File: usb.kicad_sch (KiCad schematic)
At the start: 17 parts, among them J3 USB_C_Receptacle_USB2.0_14P, J4 USB_C_Receptacle_USB2.0_14P, J5 USB_C_Receptacle_USB2.0_14P, U1 ECP5U_12_CABGA256, U5 TPD2EUSB30, U6 TPD2EUSB30, U7 FT231XQ, U8 TPD2EUSB30

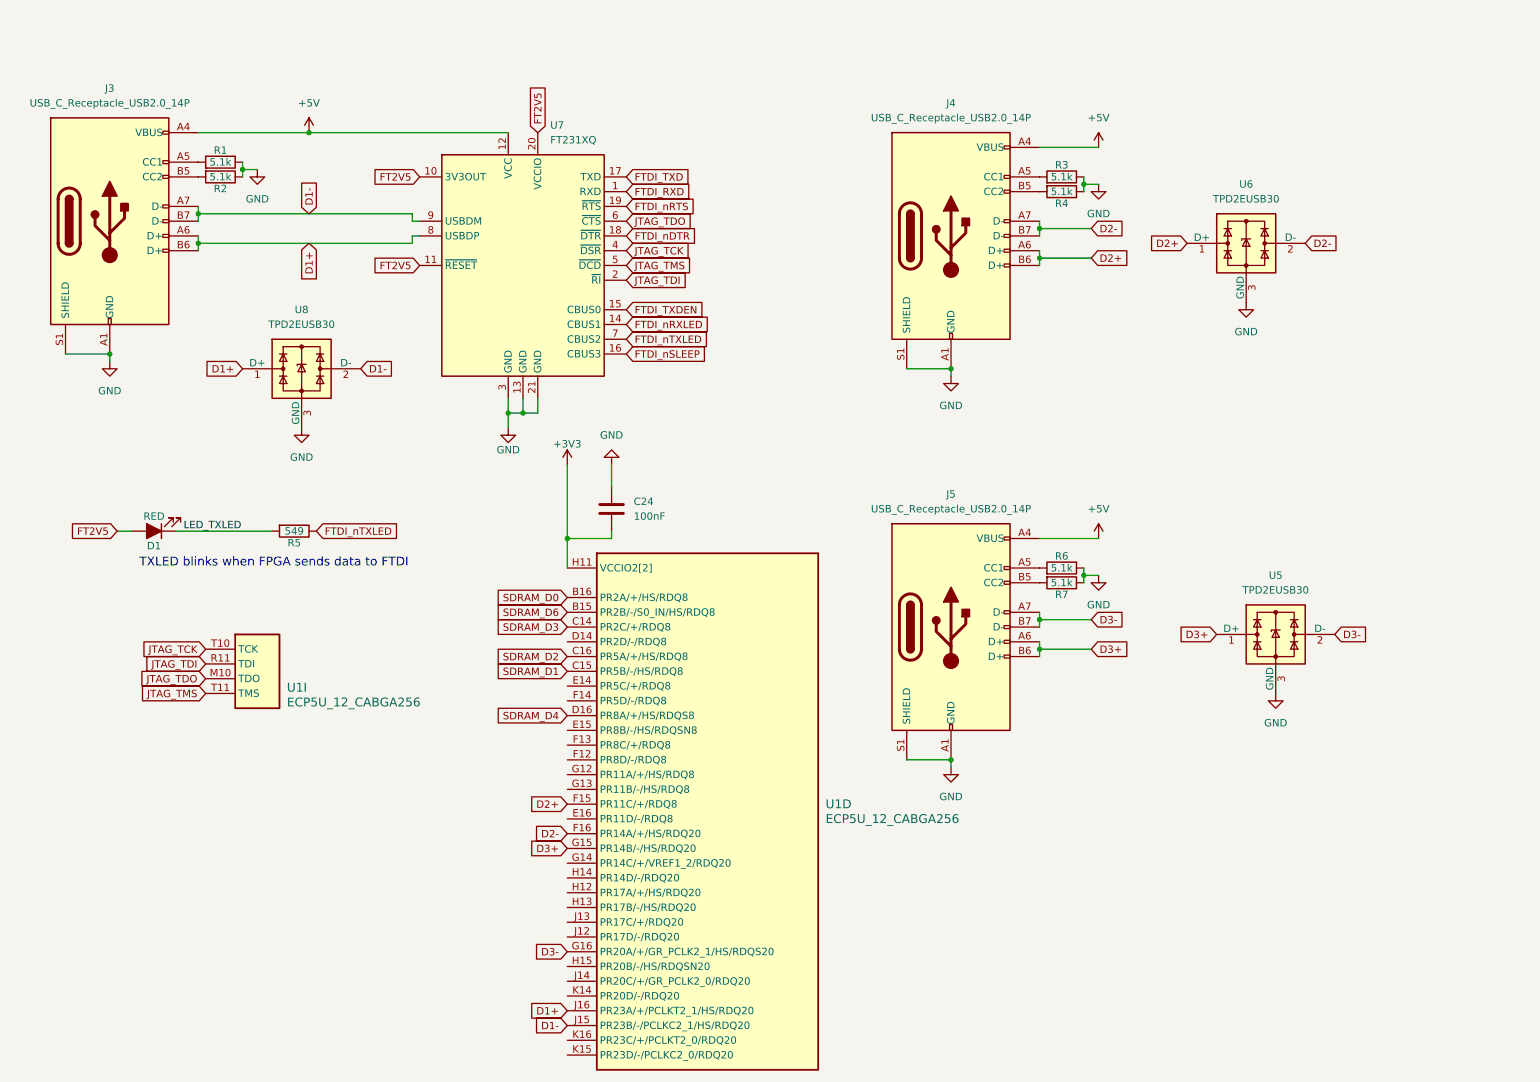
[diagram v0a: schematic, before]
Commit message: Stash
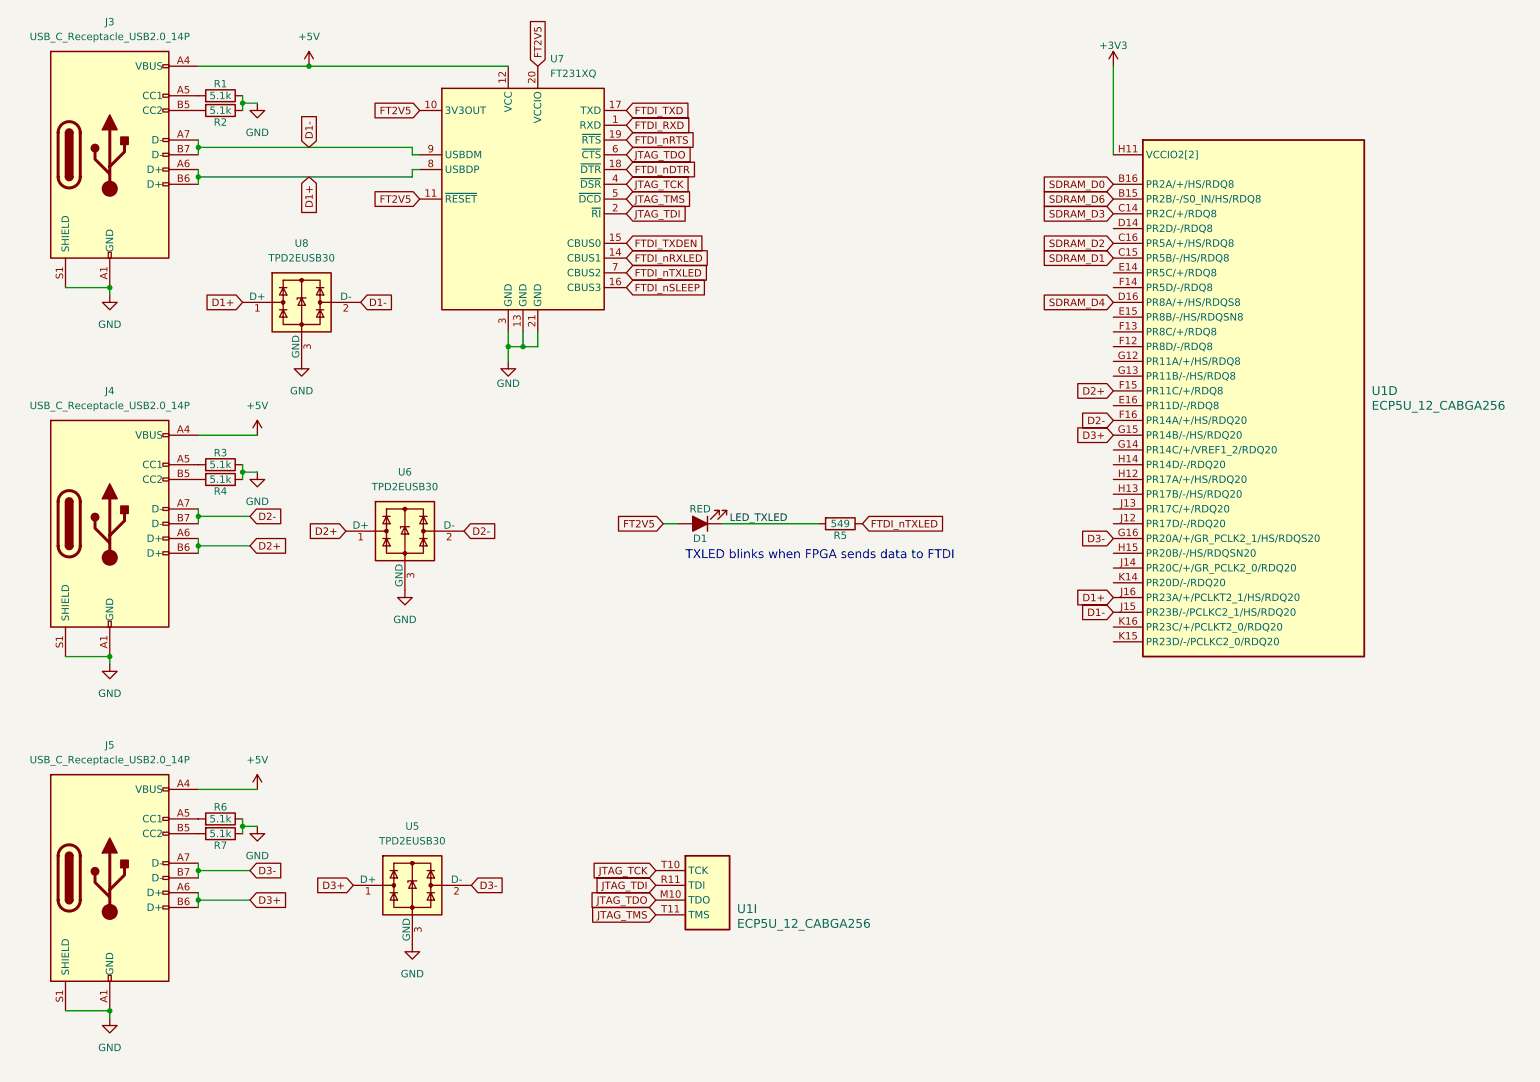
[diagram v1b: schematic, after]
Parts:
- removed C24: 100nF, Capacitor_SMD:C_0402_1005Metric, symbol Device:C
- D1: footprint LED_SMD:LED_0805_2012Metric -> LED_SMD:LED_0603_1608Metric
- J3, J4, J5: footprint Connector_USB:USB_C_Receptacle_Palconn_UTC16-G -> Connector_USB:USB_C_Receptacle_GCT_USB4105-xx-A_16P_TopMnt_Horizontal
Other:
- moved on the sheet: D1, J3, J4, J5, R1, R2, R3, R4, R5, R6, R7, U1D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
